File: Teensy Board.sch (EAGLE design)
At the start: 2 parts

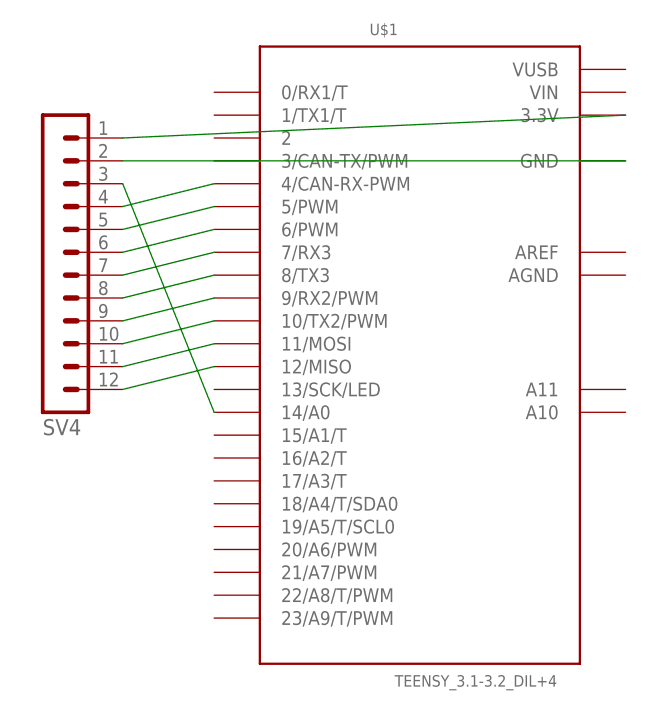
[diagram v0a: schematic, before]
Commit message: changes in Teensy Breakout Board
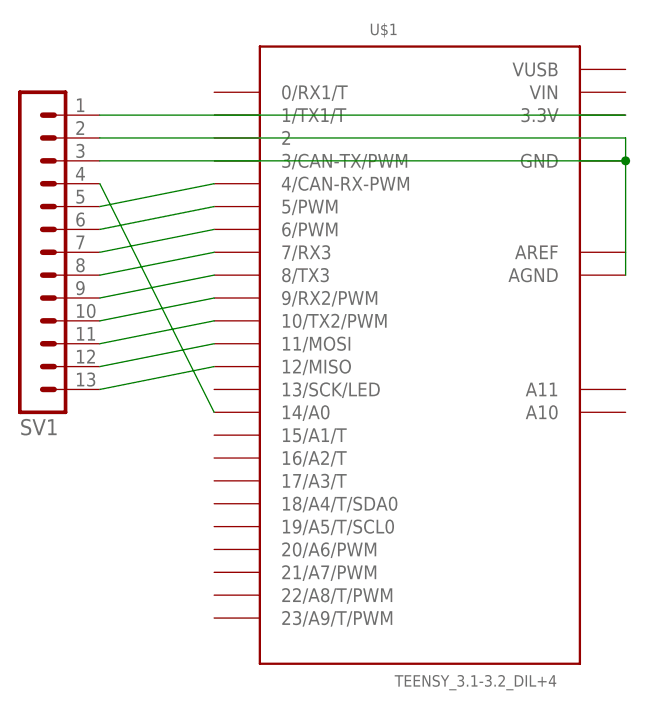
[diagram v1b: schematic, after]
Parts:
- removed SV4: (no value), con-lstb:MA12-1
- added SV1: (no value), con-lstb:MA13-1
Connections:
- net N$1: now also SV1.2, SV1.3, U$1.AGND, U$1.GND; no longer SV4.1, U$1.3.3V
- net N$10: now also SV1.6, U$1.5/PWM; no longer SV4.6, U$1.6/PWM
- net N$11: now also SV1.5, U$1.4/CAN-RX-PWM; no longer SV4.5, U$1.5/PWM
- net N$12: now also SV1.4, U$1.14/A0; no longer SV4.4, U$1.4/CAN-RX-PWM
- net N$2: now also SV1.1, U$1.3.3V; no longer SV4.2, U$1.GND
- net N$3: now also SV1.13, U$1.12/MISO; no longer SV4.3, U$1.14/A0
- net N$4: now also SV1.12, U$1.11/MOSI; no longer SV4.12, U$1.12/MISO
- net N$5: now also SV1.11, U$1.10/TX2/PWM; no longer SV4.11, U$1.11/MOSI
- net N$6: now also SV1.10, U$1.9/RX2/PWM; no longer SV4.10, U$1.10/TX2/PWM
- net N$7: now also SV1.9, U$1.8/TX3; no longer SV4.9, U$1.9/RX2/PWM
- net N$8: now also SV1.8, U$1.7/RX3; no longer SV4.8, U$1.8/TX3
- net N$9: now also SV1.7, U$1.6/PWM; no longer SV4.7, U$1.7/RX3
